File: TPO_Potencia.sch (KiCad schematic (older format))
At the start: 25 parts

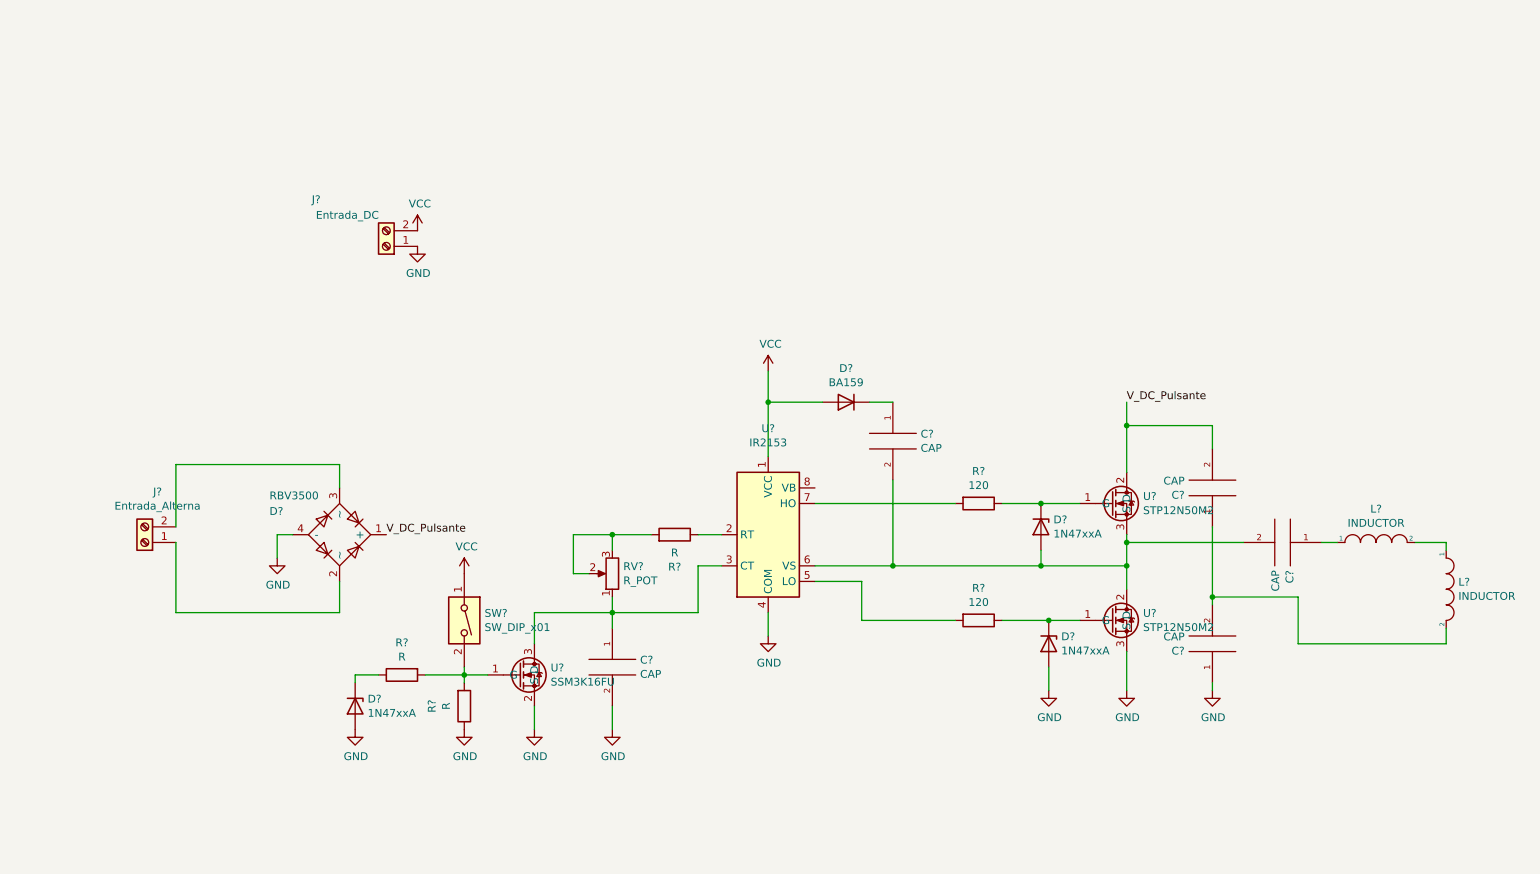
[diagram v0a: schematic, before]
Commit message: Esquematico terminado, falta asignar footprints correspondientes
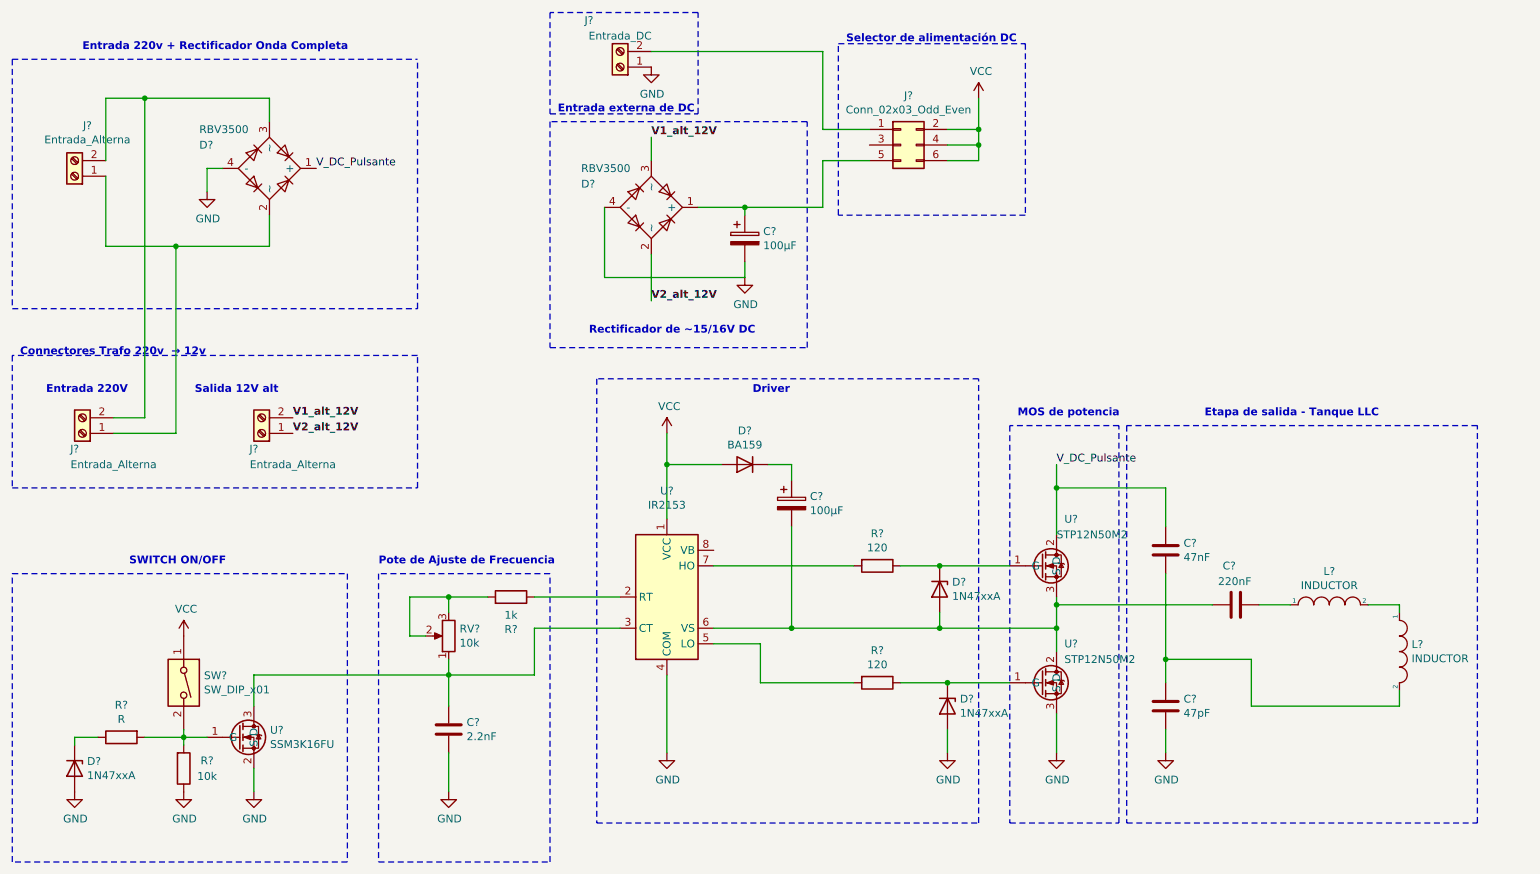
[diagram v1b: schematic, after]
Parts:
- removed C? (x5): CAP, symbol pspice:CAP
- added C?: 47nF, symbol Device:C
- added C?: 47pF, symbol Device:C
- added C?: 220nF, symbol Device:C
- added C?: 2.2nF, symbol Device:C
- added C? (x2): 100µF, symbol Device:CP
- added D?: RBV3500, symbol Diode_Bridge:RBV3500
- added J?: Conn_02x03_Odd_Even, symbol Connector_Generic:Conn_02x03_Odd_Even
- added J? (x2): Entrada_Alterna, symbol Connector:Screw_Terminal_01x02
- R?: value R -> 1k
- R?: value R -> 10k
- RV?: value R_POT -> 10k
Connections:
- net GND: now also C?.2, C?.2, C?.2, D?.4 (-)
- net VCC: now also J?.2 (Pin_2), J?.4 (Pin_4), J?.6 (Pin_6); no longer J?.2 (Pin_2)
- net V_DC_Pulsante: now also C?.1
- net at D?.2 (~~), J?.1 (Pin_1): now also J?.1 (Pin_1)
- net at D?.3 (~~), J?.2 (Pin_2): now also J?.2 (Pin_2)
- net at RV?.1, U?.3 (CT), U?.3 (D): now also C?.1
- net at D?.2 (A), U?.2 (D), U?.3 (S)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: now also C?.1, C?.2
- net at L?.1: now also C?.2
- net at L?.2: now also C?.1, C?.2
- net at D?.1 (K): now also C?.1
- new net: J?.1 (Pin_1), J?.2 (Pin_2)
- new net: C?.1, D?.1 (+), J?.5 (Pin_5)
- new net V1_alt_12V: D?.3 (~~), J?.2 (Pin_2)
- new net V2_alt_12V: D?.2 (~~), J?.1 (Pin_1)
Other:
- note added: "Connectores Trafo 220v → 12v\n\n\n Entrada 220V Salida 12V alt\n"
- note added: "Driver\n"
- note added: "Entrada 220v + Rectificador Onda Completa\n"
- note added: "Entrada externa de DC\n"
- note added: "Etapa de salida - Tanque LLC\n"
- note added: "MOS de potencia\n"
- note added: "Pote de Ajuste de Frecuencia\n"
- note added: "Rectificador de ~~15/16V DC\n\n"
- note added: "SWITCH ON/OFF"
- note added: "Selector de alimentación DC\n"
- moved on the sheet: D?, J?, L?, R?, RV?, SW?, U?
